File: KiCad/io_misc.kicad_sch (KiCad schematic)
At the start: 0 parts

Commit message: feat: add sd + gps+ swd + LED RG + add sma
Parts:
- added C37, C45: 100nF, ODB:C_0402_1005Metric, symbol Device:C_Small
- added D13: LTST-E682KRKGWT, ODB:LTSTE683RGBW, symbol ODB2:LTST-E682KRKGWT
- added J1: SMA-50G, CONN_142-0701-801, symbol PayloadLibrary:SMA-50G
- added J2: MEM2067-02-180-00-A_REVB, MEM2067-02-180-00-A_REVB:GCT_MEM2067-02-180-00-A_REVB, symbol PayloadLibrary:MEM2067-02-180-00-A_REVB
- added J7: SYS_SW_Conn_01x05_Header, Connector_PinHeader_2.54mm:PinHeader_1x05_P2.54mm_Vertical, symbol ODB2:705430004
- added L1: 100nH, Inductor_SMD:L_0603_1608Metric, symbol Device:L
- added R3: 10R, ODB:R_0402_1005Metric, symbol Device:R
- added R30: 22R, ODB:R_0402_1005Metric, symbol Device:R
- added R32, R33: 100R, Resistor_SMD:R_0603_1608Metric, symbol Device:R
- added R51: 10k, Resistor_SMD:R_0603_1608Metric, symbol Device:R
- added U5: L76L-M33, L76L-M33:XCVR_L76L-M33, symbol PayloadLibrary:L76L-M33
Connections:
- new net: D13.4 (A_GREEN), R33.1
- new net: J2.10 (SHIELD__1), J2.11 (SHIELD__2), J2.12 (SHIELD__3), J2.9 (SHIELD)
- new net: J2.7 (DAT0), R30.2
- new net: L1.1, R3.1
- new net: R3.2, U5.14 (VCC_RF)
- new net: D13.2 (A_RED), R32.2
- new net +3V3: C37.1, C45.1, J2.4 (VDD), J7.3, R32.1, R33.2, R51.1, U5.6 (V_BCKP), U5.8 (VCC)
- new net CriticalLED_G: D13.3 (K_GREEN)
- new net CriticalLED_R: D13.1 (K_RED)
- new net GND: C37.2, C45.2, J1.2 (SHIELD), J1.3 (SHIELD), J1.4 (SHIELD), J1.5 (SHIELD), J2.6 (VSS), J7.5, R51.2, U5.1 (GND), U5.10 (GND__1), U5.12 (GND__2), U5.9 (RESET)
- new net GPS_USART6_RX: U5.2 (TXD1)
- new net GPS_USART6_TX: U5.3 (RXD1)
- new net L76LM33_RF: J1.1, L1.2, U5.11 (RF_IN)
- new net SD_SPI5_CLK: J2.5 (CLK)
- new net SD_SPI5_CS: J2.2 (CD/DAT3)
- new net SD_SPI5_MISO: R30.1
- new net SD_SPI5_MOSI: J2.3 (CMD)
- new net SYS_SWCLK: J7.2
- new net SYS_SWDIO: J7.1
- new net SYS_SWO: J7.4
- no-connect marks 0 -> 7
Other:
- note added: "CriticalLED"
- note added: "GPS"
- note added: "Max consumption ~250mA"
- note added: "Max consumption ~50mA"
- note added: "R = (3.3 - 2.0)V / 0.002A = 650R"
- note added: "SD Card"
- note added: "SYS_SW Connector"

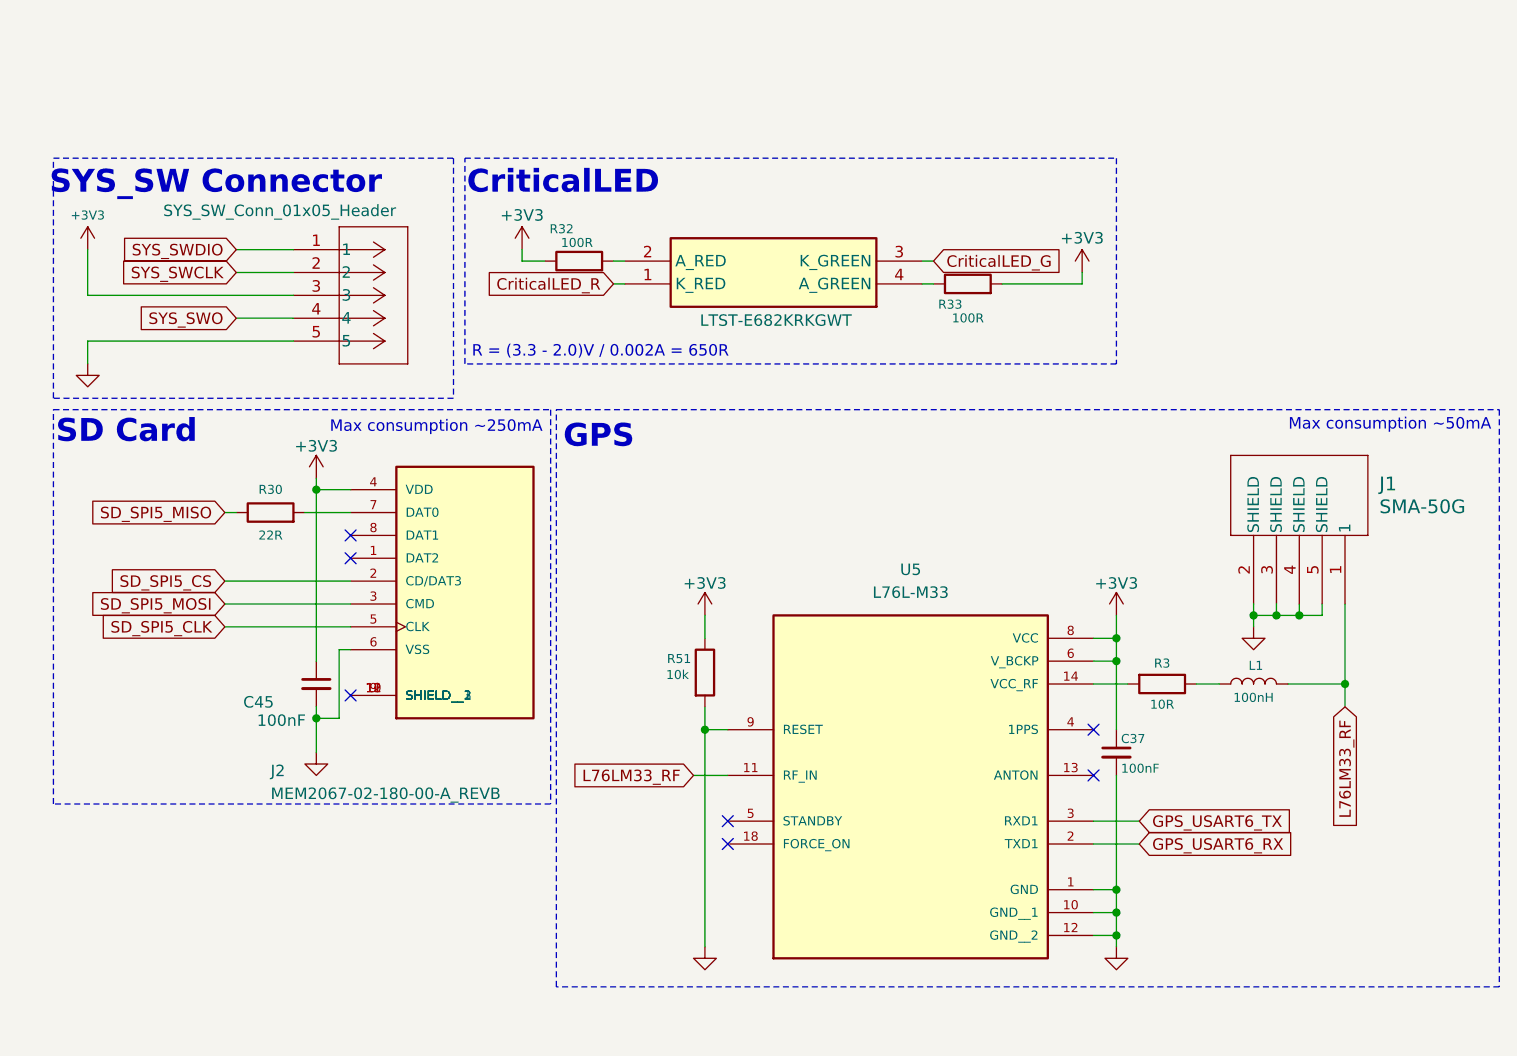
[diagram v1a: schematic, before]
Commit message: Added hardware
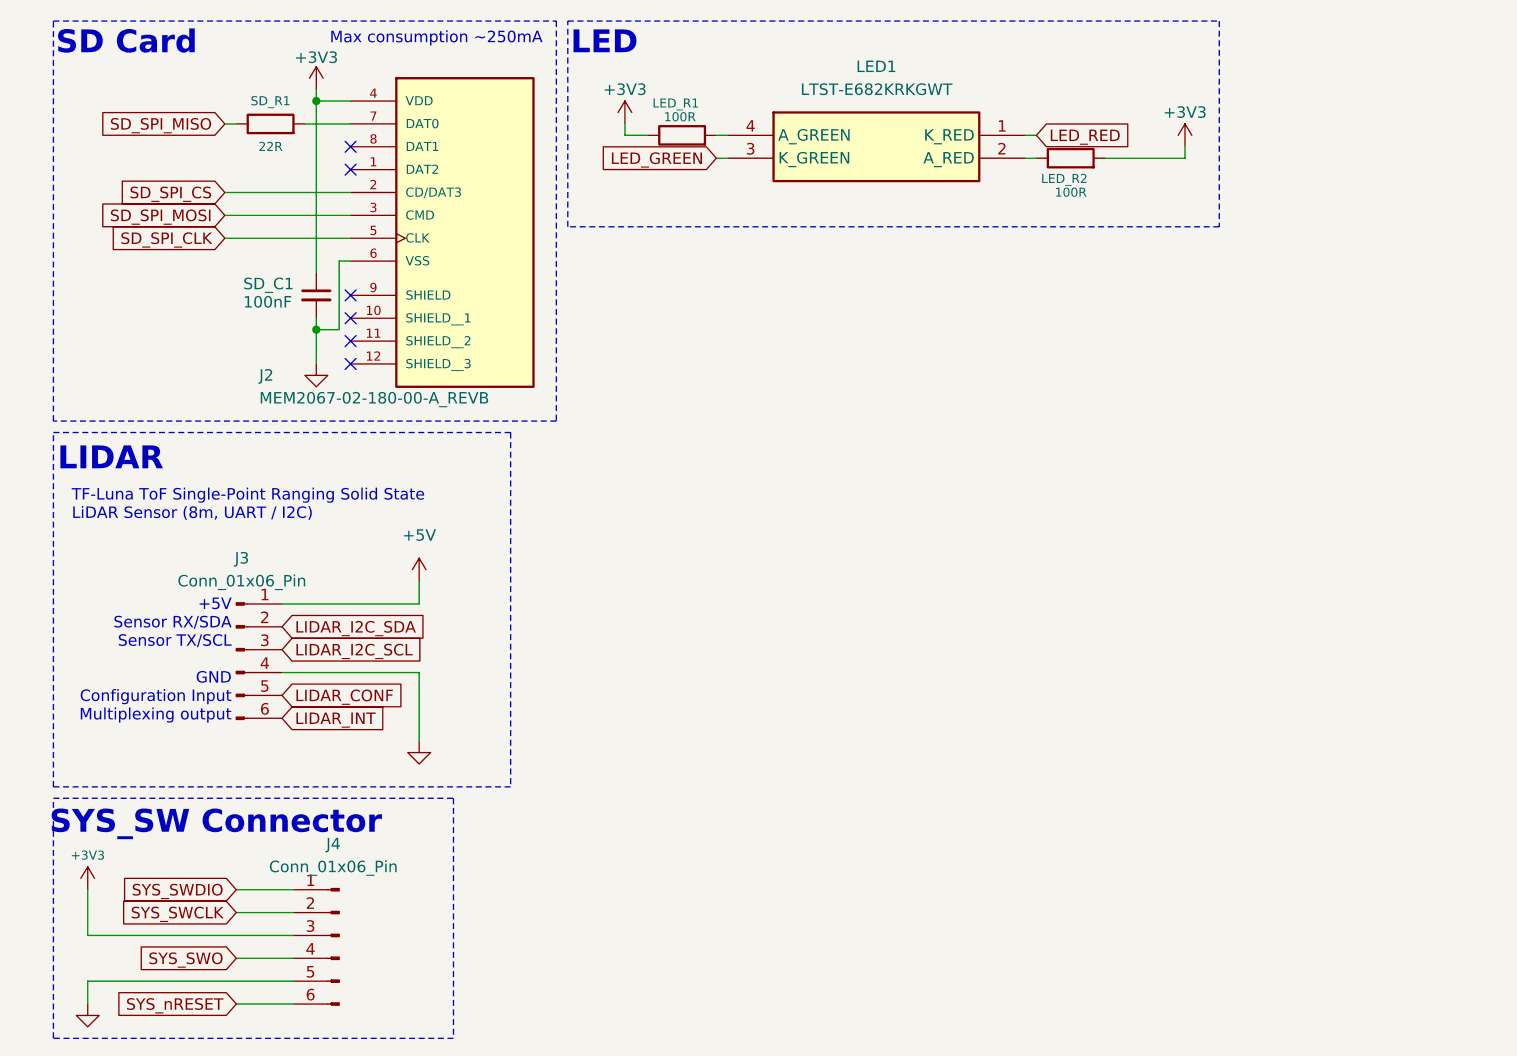
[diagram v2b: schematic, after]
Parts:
- removed C37: 100nF, ODB:C_0402_1005Metric, symbol Device:C_Small
- removed D13: LTST-E682KRKGWT, ODB:LTSTE683RGBW, symbol ODB2:LTST-E682KRKGWT
- removed J1: SMA-50G, CONN_142-0701-801, symbol PayloadLibrary:SMA-50G
- removed J7: SYS_SW_Conn_01x05_Header, Connector_PinHeader_2.54mm:PinHeader_1x05_P2.54mm_Vertical, symbol ODB2:705430004
- removed L1: 100nH, Inductor_SMD:L_0603_1608Metric, symbol Device:L
- removed R3: 10R, ODB:R_0402_1005Metric, symbol Device:R
- removed R51: 10k, Resistor_SMD:R_0603_1608Metric, symbol Device:R
- removed U5: L76L-M33, L76L-M33:XCVR_L76L-M33, symbol PayloadLibrary:L76L-M33
- added J3, J4: Conn_01x06_Pin, Connector_PinHeader_2.54mm:PinHeader_1x06_P2.54mm_Vertical, symbol Connector:Conn_01x06_Pin
- added LED1: LTST-E682KRKGWT, LTSTE683RGBW, symbol PayloadLibrary:LTST-E682KRKGWT
- renumbered R32 to LED_R1, R33 to LED_R2, C45 to SD_C1, R30 to SD_R1
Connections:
- net +3V3: now also J4.3 (Pin_3)
- net GND: now also J3.4 (Pin_4), J4.5 (Pin_5)
- net SYS_SWCLK: now also J4.2 (Pin_2)
- net SYS_SWDIO: now also J4.1 (Pin_1)
- net SYS_SWO: now also J4.4 (Pin_4)
- net at LED_R2.1: now also LED1.2 (A_RED)
- net at LED_R1.2: now also LED1.4 (A_GREEN)
- net SD_SPI5_CLK renamed SD_SPI_CLK
- net SD_SPI5_CS renamed SD_SPI_CS
- net SD_SPI5_MISO renamed SD_SPI_MISO
- net SD_SPI5_MOSI renamed SD_SPI_MOSI
- new net +5V: J3.1 (Pin_1)
- new net LED_GREEN: LED1.3 (K_GREEN)
- new net LED_RED: LED1.1 (K_RED)
- new net LIDAR_CONF: J3.5 (Pin_5)
- new net LIDAR_I2C_SCL: J3.3 (Pin_3)
- new net LIDAR_I2C_SDA: J3.2 (Pin_2)
- new net LIDAR_INT: J3.6 (Pin_6)
- new net SYS_nRESET: J4.6 (Pin_6)
- now unconnected: J2.10 (SHIELD__1), J2.11 (SHIELD__2), J2.12 (SHIELD__3), J2.9 (SHIELD)
- no-connect marks 7 -> 6
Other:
- note added: "+5V Sensor RX/SDA Sensor TX/SCL GND Configuration Input Multiplexing output"
- note added: "LED"
- note added: "LIDAR"
- note added: "TF-Luna ToF Single-Point Ranging Solid State LiDAR Sensor (8m, UART / I2C)"
- note removed: "CriticalLED"
- note removed: "GPS"
- note removed: "Max consumption ~50mA"
- note removed: "R = (3.3 - 2.0)V / 0.002A = 650R"
- moved on the sheet: LED_R1, LED_R2, SD_C1, SD_R1
